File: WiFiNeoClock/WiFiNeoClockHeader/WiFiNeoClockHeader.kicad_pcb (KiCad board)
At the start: 2 copper layers, 68.6 x 73.7 mm, 9 parts, among them P1 CONN_01X10, P2 CONN_01X10, P3 CONN_01X03, SW1 SW_PUSH, SW2 Switch_SPDT_x2

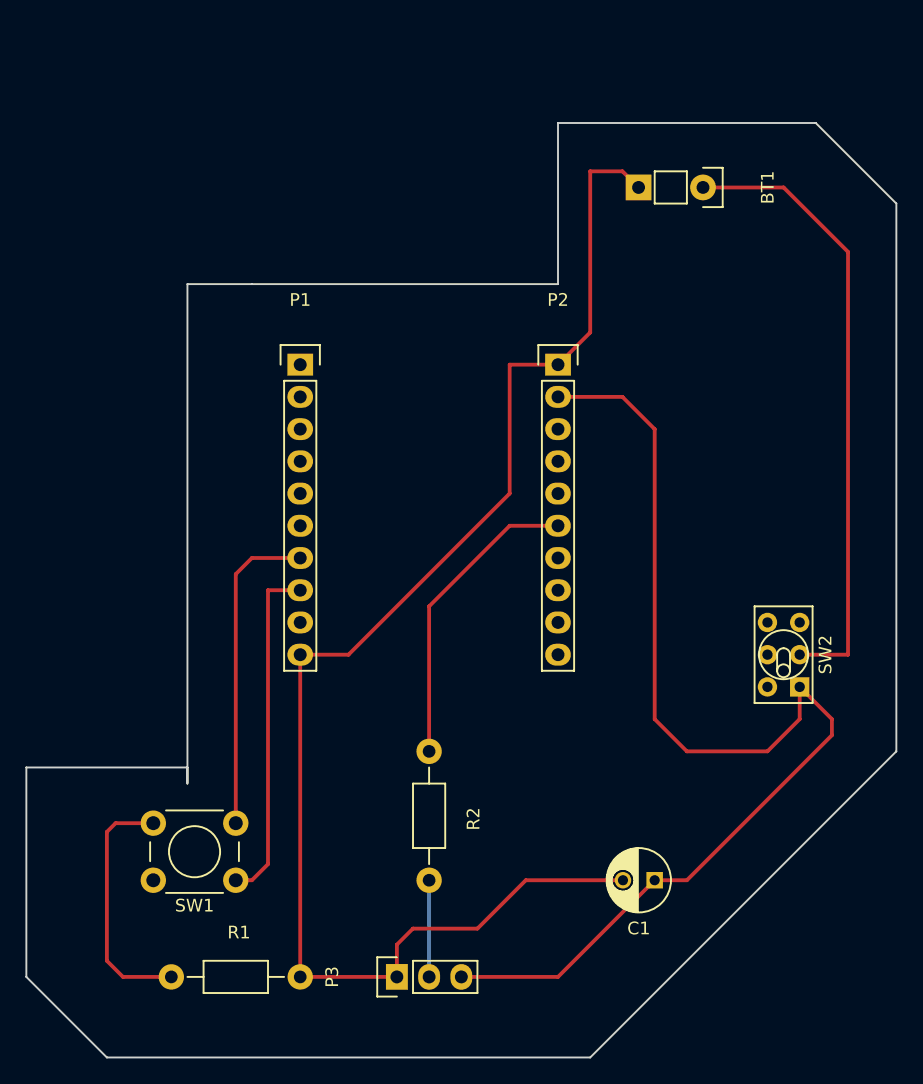
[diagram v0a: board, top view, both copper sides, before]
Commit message: Signed-off-by: Edith Li <abenoy05@gmail.com>
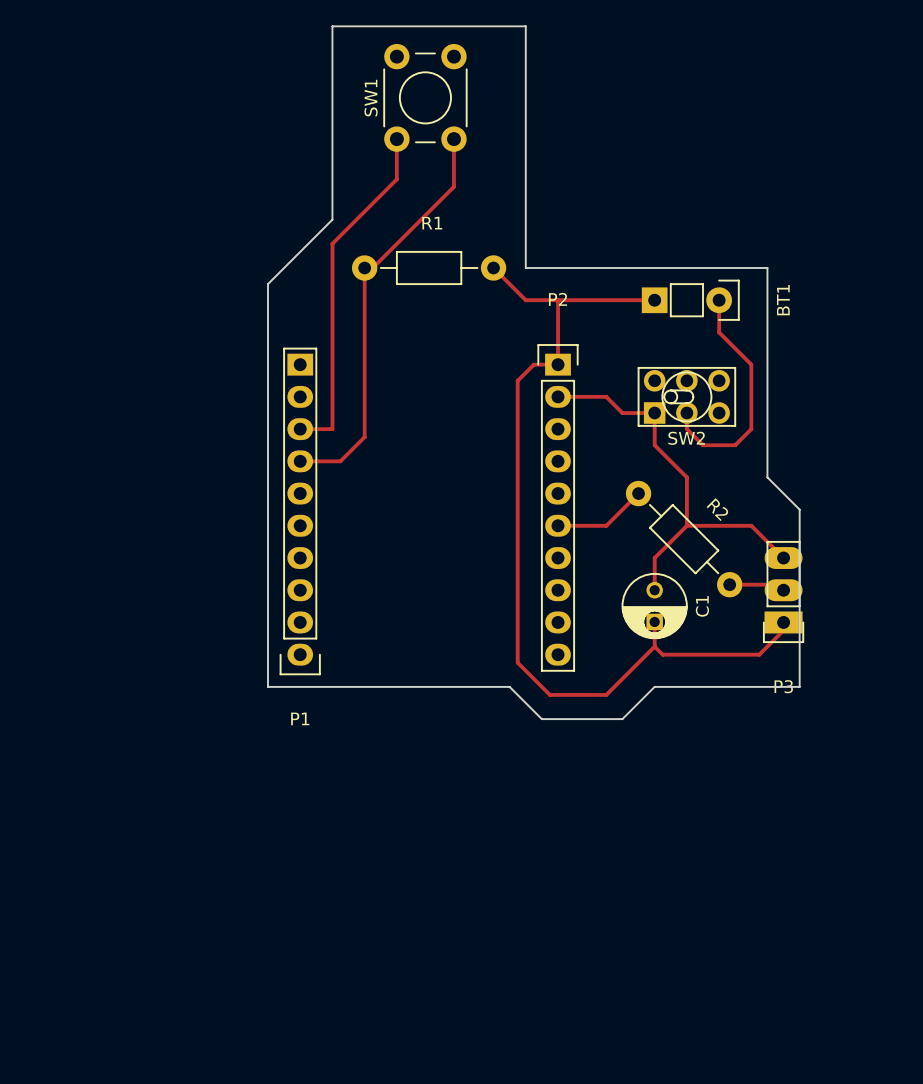
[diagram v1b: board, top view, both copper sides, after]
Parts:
- moved SW1 59.8 mm to (124.5, 61.0), turned to 90 degrees
- moved R1 57.9 mm to (121.9, 71.1)
- moved P3 41.3 mm to (154.9, 99.1), turned to 180 degrees
- moved R2 26.2 mm to (143.5, 88.9), turned to 315 degrees
- moved C1 22.9 mm to (144.8, 96.5), turned to 270 degrees
- moved P1 22.9 mm to (116.8, 101.6), turned to 180 degrees
- moved SW2 21.7 mm to (147.3, 81.3), turned to 0 degrees
- moved BT1 8.98 mm to (149.9, 73.7)
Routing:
- net VBat: track 89.6 -> 33.5 mm
- net GND: track 111.9 -> 72.0 mm
- net Net-(BT1-Pad1): track 49.1 -> 18.6 mm
- net 14: track 24.2 -> 7.40 mm
- net 15: track 44.9 -> 32.7 mm
- net Net-(P3-Pad2): track 7.62 -> 4.43 mm
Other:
- board size 68.6 x 73.7 mm -> 41.9 x 54.6 mm
